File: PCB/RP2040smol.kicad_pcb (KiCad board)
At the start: 4 copper layers, 25 x 25 mm, 40 parts, among them SW1 BOOTSEL, SW2 RESET, U1 AP2112K-3.3, U2 RP2040, U3 W25Q64JVZP, Y1 Crystal_520-120-18-33JGN-TR3

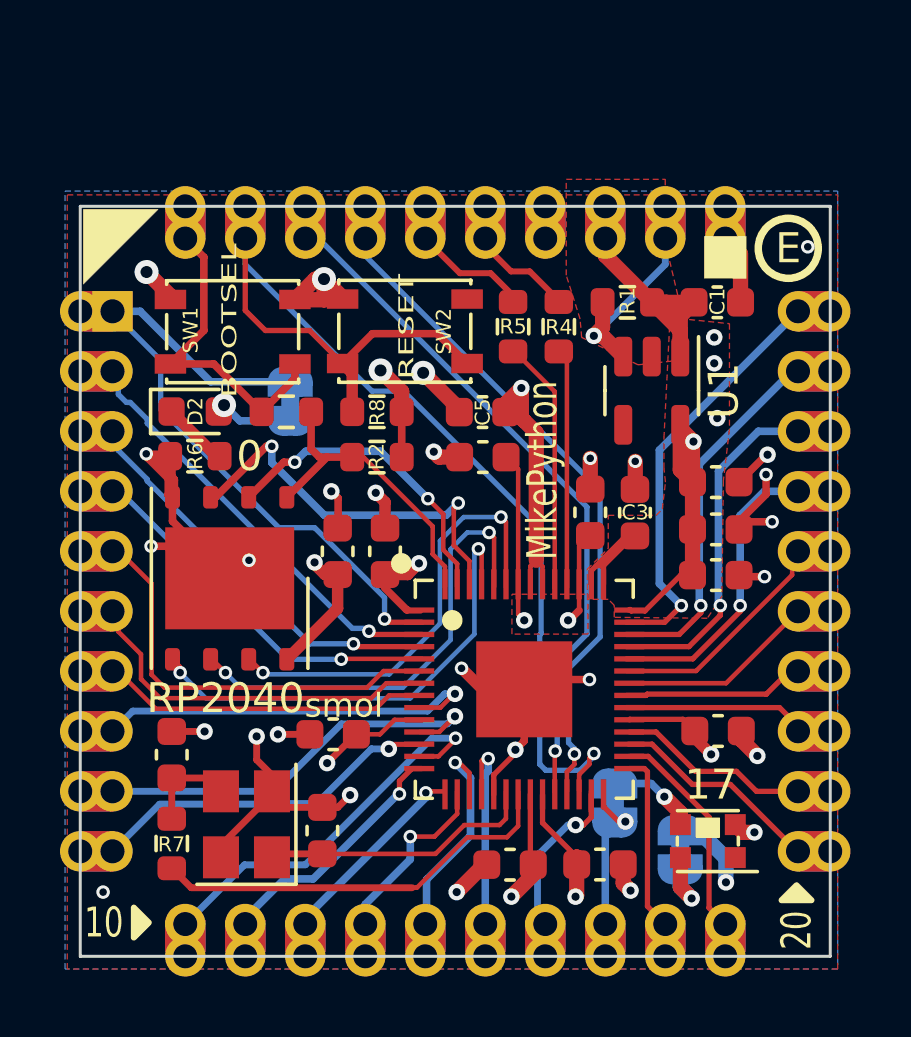
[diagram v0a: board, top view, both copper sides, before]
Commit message: m
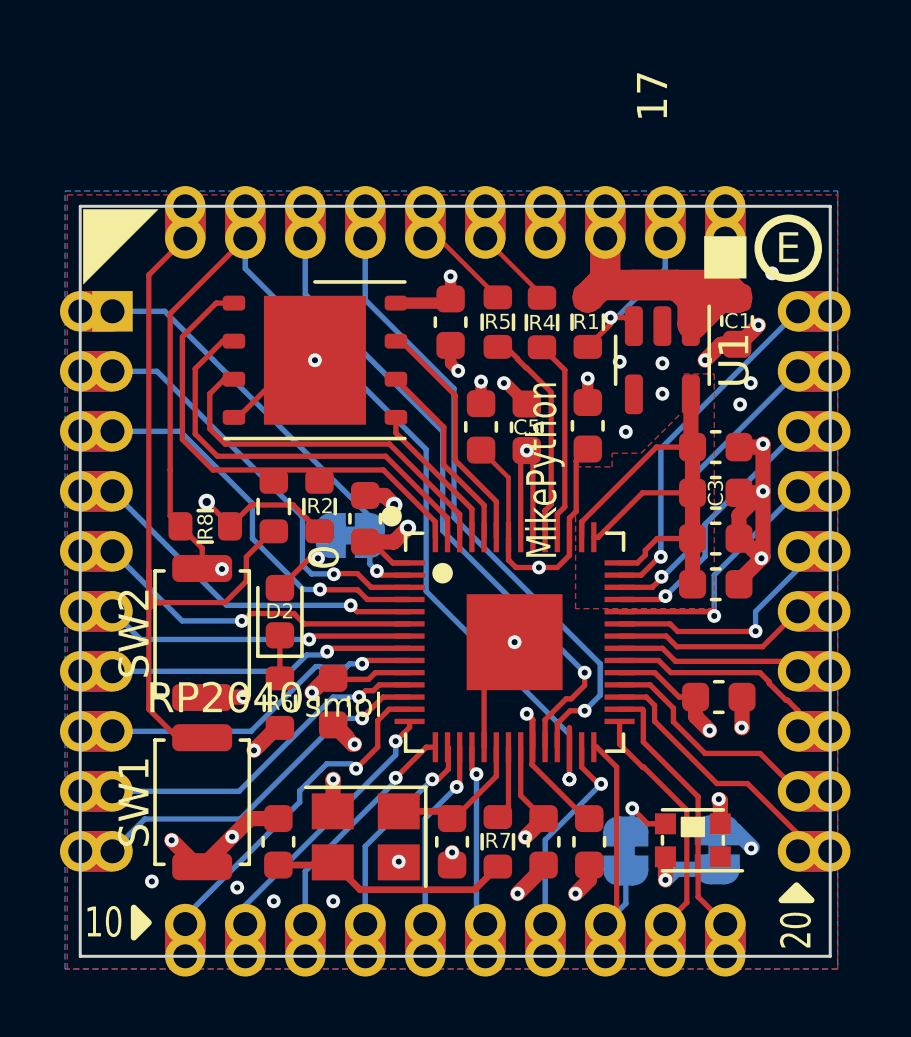
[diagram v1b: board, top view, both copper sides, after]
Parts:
- SW1, SW2: footprint Button_Switch_SMD:SW_SPST_PTS810 -> MikeSwitchFootprints:SW_Push_SPST_Alps_SKRK_Clone
- moved SW1 15.7 mm to (130.6, 116.4), turned to 90 degrees
- moved SW2 12.1 mm to (130.6, 110.7), turned to 90 degrees
- moved R7 10.9 mm to (140.4, 117.7), turned to -90 degrees
- moved R6 8.71 mm to (133.2, 113.1), turned to 90 degrees
- moved C14 8.52 mm to (138.8, 100.4), turned to -90 degrees
- moved U3 7.81 mm to (134.3, 101.6), turned to 0 degrees
- moved D2 7.25 mm to (133.2, 110.0), turned to 90 degrees
- moved R8 6.88 mm to (130.7, 107.2)
- moved JP3 4.90 mm to (135.5, 107.5), turned to 180 degrees
- moved C16 4.59 mm to (133.1, 117.7)
- moved C15 4.34 mm to (138.9, 117.7), turned to -90 degrees
- moved Y1 4.00 mm to (136.0, 117.5), turned to 180 degrees
- moved R3 3.19 mm to (133.0, 106.5), turned to -90 degrees
- moved C10 2.89 mm to (143.4, 103.8)
- moved C3 2.77 mm to (147.7, 106.1), turned to 180 degrees
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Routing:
- net /BOOTSEL: track 10.7 -> 25.3 mm
- net GND: track 50.2 -> 38.7 mm, vias 28 -> 35
- net /XOUT: track 13.9 -> 2.48 mm
- net /QSPI_SD0: track 15.8 -> 5.04 mm, vias 2 -> 0
- net +1V1: track 25.9 -> 15.8 mm, vias 3 -> 2
- net /QSPI_SCLK: track 15.4 -> 6.48 mm, vias 2 -> 0
- net /GPIO0: track 22.4 -> 15.5 mm
- net /QSPI_SD3: track 14.8 -> 8.02 mm, vias 2 -> 0
- net /QSPI_SS: track 10.5 -> 15.7 mm
- net Net-(C16-Pad2): track 3.18 -> 8.05 mm
- net /GPIO17: track 4.00 -> 8.50 mm, vias 1 -> 0
- net /XIN: track 9.08 -> 4.91 mm
- net /QSPI_SD1: track 10.6 -> 14.1 mm, vias 2 -> 0
- net +5V: track 9.49 -> 12.4 mm
- net /GPIO29_ADC3: track 14.6 -> 11.7 mm
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- removed copper zone on F.Cu, net +1V1
- removed copper zone on F.Cu, net +5V
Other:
- board text added: "Compatible with Rev E solder stencil"
- board text removed: "Compatible with Rev D solder stencil"
